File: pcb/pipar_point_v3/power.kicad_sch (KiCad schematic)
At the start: 24 parts, among them J1 USB_C_Receptacle_USB2.0_16P, J5 Conn_01x02, SW5 SW_SPDT, U11 nPM1300-QEXX, U4 ESDR0502NMUTAG

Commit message: Update pipar_point_v3.zip with latest production files
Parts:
- U11: Manufacturer_Part_Number (none) -> nPM1300-QEAA-R7; Mouser Part Number (none) -> 949-NPM1300-QEAA-R7
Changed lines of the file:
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@@
+			)
+		)
+		(property "Manufacturer_Part_Number" "nPM1300-QEAA-R7"
+			(at 168.91 77.47 0)
+			(effects
+				(font
+					(size 1.27 1.27)
+				)
+				(hide yes)
+			)
+		)
+		(property "Mouser Part Number" "949-NPM1300-QEAA-R7"
+			(at 168.91 77.47 0)
+			(effects
+				(font
+					(size 1.27 1.27)
+				)
+				(hide yes)
 			)
 		)

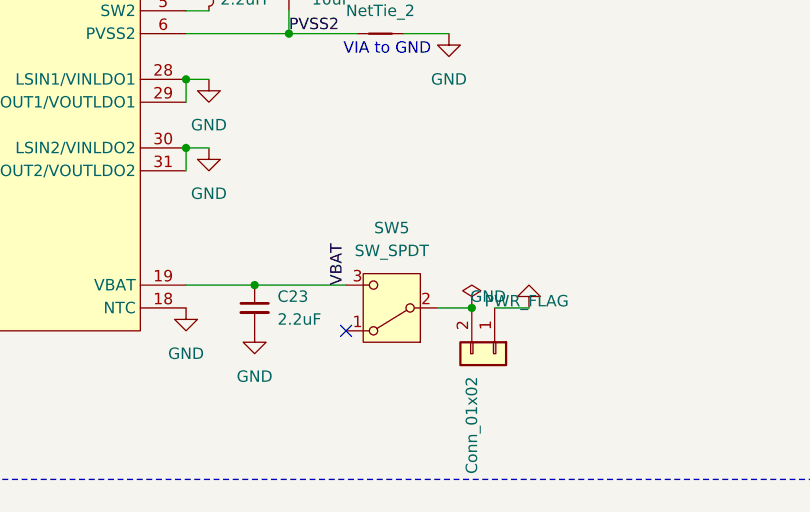
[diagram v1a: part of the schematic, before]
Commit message: Pipar Point V3.1
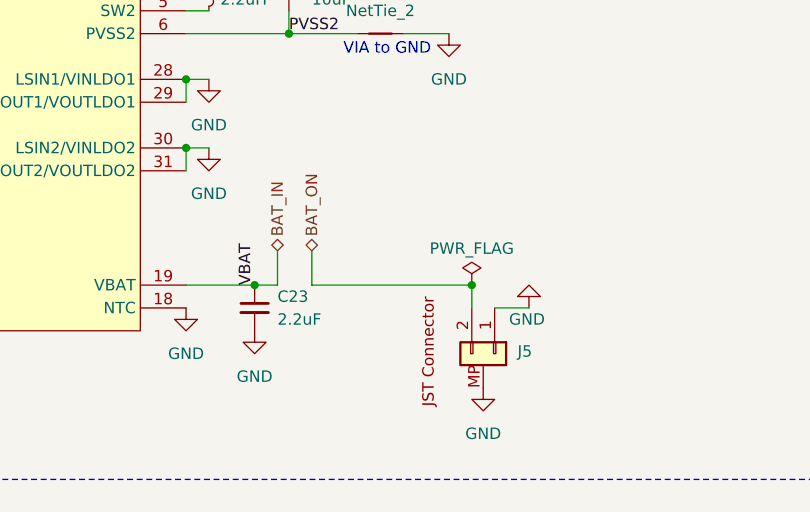
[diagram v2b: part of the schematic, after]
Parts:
- removed J5: Conn_01x02, Connector_JST:JST_PH_S2B-PH-SM4-TB_1x02-1MP_P2.00mm_Horizontal, symbol Connector_Generic:Conn_01x02
- removed SW5: SW_SPDT, Button_Switch_SMD:SW_SPDT_PCM12, symbol Switch:SW_SPDT
- added J5: Conn_JST_PH_S2B-PH-SM4-TB_1x02-1MP_P2.00mm_Horizo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, Connector_JST:JST_PH_S2B-PH-SM4-TB_1x02-1MP_P2.00mm_Horizontal, symbol Keyboard:Conn_JST_PH_S2B-PH-SM4-TB_1x02-1MP_P2.00mm_Horizontal
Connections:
- net GND: now also J5.1 (Pin_1), J5.MP
- net VBAT renamed BAT_IN
- new net BAT_ON: J5.2 (Pin_2)
- no-connect marks 11 -> 10
